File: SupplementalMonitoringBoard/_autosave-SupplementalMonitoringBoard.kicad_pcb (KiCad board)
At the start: 2 copper layers, 53.5 x 77 mm, 47 parts, among them J1 PeripheralCANConnector, J2 PeripheralCANConnector, U1 OPA842xDBV, U2 OPA842xDBV, U3 INA180B1, U4 PAMC131M03QDFMRQ1, U5 PeripheralSOM

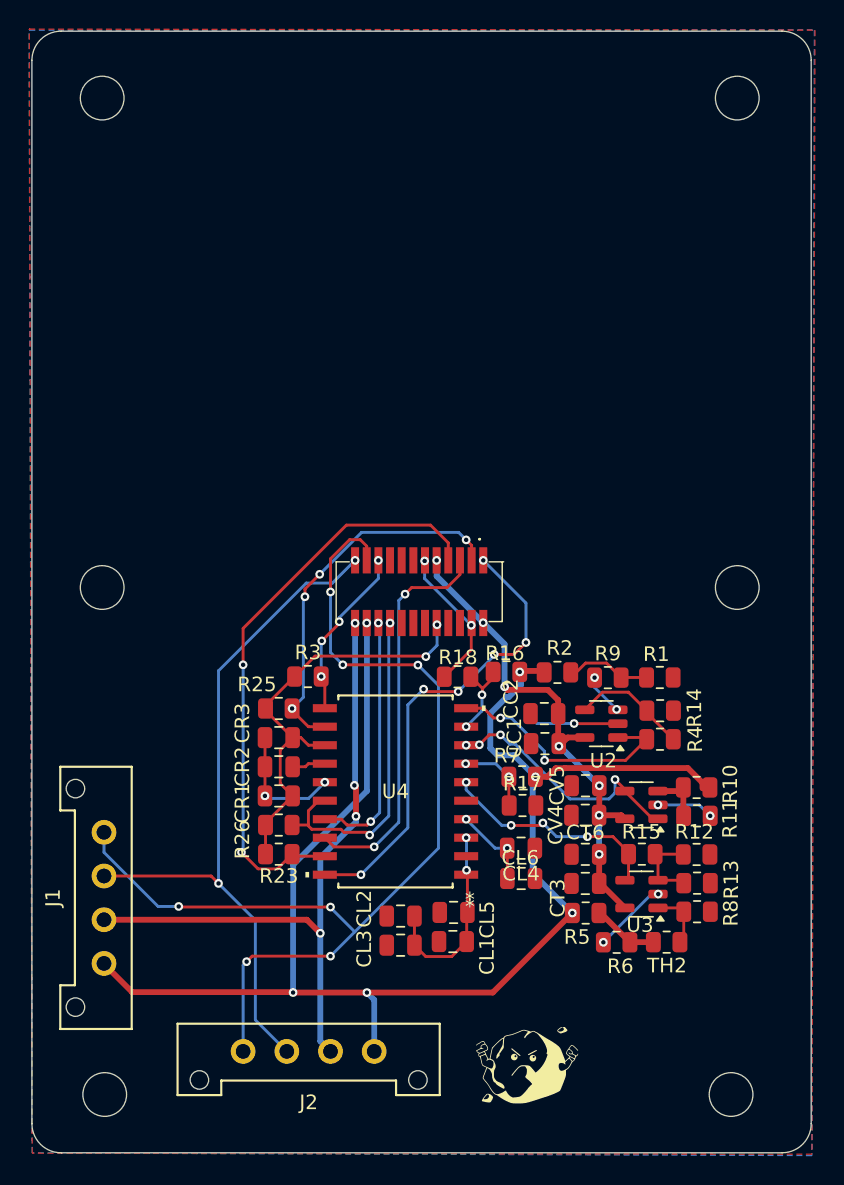
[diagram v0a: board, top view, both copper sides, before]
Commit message: Supplemental MOnitoring Board
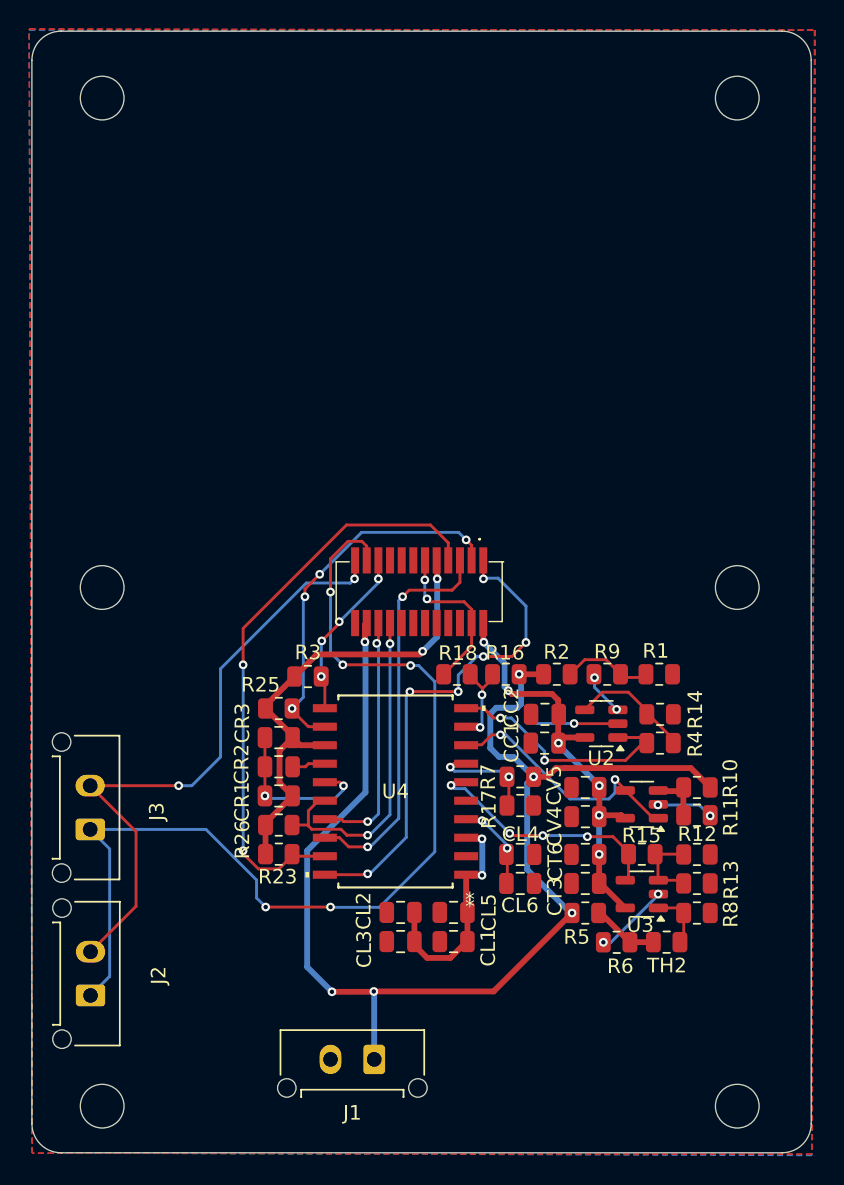
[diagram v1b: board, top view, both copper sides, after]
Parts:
- removed the ? at (124.5, 129.0)
- removed the ? at (167.5, 129.0)
- removed G***: LOGO, LOGO
- added ?: , , F.Cu at (167.9, 129.8)
- added ?: , , F.Cu at (124.3, 129.8)
- added J3: CANconn2, Connector_Molex:Molex_Micro-Fit_3.0_43650-0215_1x02_P3.00mm_Vertical, F.Cu at (123.5, 110.8)
- CC1, CT3, CV5: value .1uF -> 1nF
- CL2, CL5, CL6, CR1: value 1nF -> .1uF
- J1: value PeripheralCANConnector -> CarPowerConnector; footprint UTSVT_Connectors:Molex_MicroFit3.0_1x4xP3.00mm_PolarizingPeg_Vertical -> Connector_Molex:Molex_Micro-Fit_3.0_43650-0215_1x02_P3.00mm_Vertical
- J2: value PeripheralCANConnector -> CANconn; footprint UTSVT_Connectors:Molex_MicroFit3.0_1x4xP3.00mm_PolarizingPeg_Vertical -> Connector_Molex:Molex_Micro-Fit_3.0_43650-0215_1x02_P3.00mm_Vertical
- R14: value 150K -> 150k
- R2: value 50K -> 50k
- R4: value 10K -> 10k
- R7: value 30K -> 30k
- TH2: value 500 -> 500.
- moved J2 19.8 mm to (123.5, 122.2), turned to 90 degrees
- moved J1 19.7 mm to (143.0, 126.6), turned to 180 degrees
- moved CL4 0.43 mm to (153.0, 112.5)
- moved CL6 0.35 mm to (153.0, 114.5)
- moved R4 0.27 mm to (162.6, 104.9)
- moved R14 0.25 mm to (162.6, 102.9)
- moved CL2 0.25 mm to (144.8, 116.5)
- moved CL3 0.25 mm to (144.8, 118.5)
- moved R9 0.23 mm to (159.0, 100.2)
- moved R1 0.22 mm to (162.6, 100.2)
- moved R18 0.18 mm to (148.7, 100.2)
- moved R16 0.17 mm to (152.0, 100.2)
- moved R17 0.15 mm to (153.0, 109.2)
- moved R2 0.14 mm to (155.5, 100.2)
- moved R7 0.13 mm to (153.0, 107.2)
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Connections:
- J1 pad 1: +BATT -> +12V
- J1 pad 2: GNDPWR -> GND
- J2 pad 1: +BATT -> /CAN_L
- J2 pad 2: GNDPWR -> /CAN_H
- R10 pad 2: +BATT -> +12V
- R16 pad 2: +BATT -> +12V
- R2 pad 2: +BATT -> +12V
- R5 pad 2: +BATT -> +12V
- R7 pad 2: +BATT -> +12V
- U5 pad 10: /DVDD -> unconnected-(U5-VDDA(3.3V)-Pad10)
- U5 pad 22: +BATT -> +12V
- U5 pad 9: +3.3V -> /DVDD
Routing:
- net +BATT: track 102.5 -> 0.00 mm, vias 6 -> 0
- net +12V: track 0.00 -> 87.0 mm, vias 0 -> 6
- net GNDPWR: track 46.0 -> 0.00 mm, vias 4 -> 0
- net /CAN_H: track 48.7 -> 42.9 mm
- net +3.3V: track 34.8 -> 29.3 mm, vias 7 -> 6
- net GND: track 34.1 -> 38.1 mm
- net /DVDD: track 29.9 -> 33.8 mm
- net /CAN_L: track 73.7 -> 70.9 mm, vias 7 -> 5
- net /DCDC_OUT: track 13.5 -> 15.8 mm
- net /AIN12N: track 5.35 -> 7.46 mm
- net /DIN: track 32.3 -> 34.2 mm
- net /AIN2P/GPO: track 16.0 -> 17.4 mm
- net /AINOP: track 5.34 -> 5.97 mm
- net /AIN1P: vias 4 -> 2
